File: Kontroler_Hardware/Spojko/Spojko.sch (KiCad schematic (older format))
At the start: 25 parts, among them J1 CONN_01X02, J2 CONN_01X06, P1 Raspberry_Pi, Q1 BSS138, Q2 BSS138, SW1 SW_Reset, SW2 SW_Flash, U1 ESP-12E, U6 DHT11

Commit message: Puno izmena
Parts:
- added V?: VSOURCE, symbol pspice:VSOURCE
- C1, C4, C7: symbol CP -> Spojko-rescue:CP
- C2, C3, C5, C6: symbol C -> Spojko-rescue:C
- J1: symbol CONN_01X02 -> Spojko-rescue:CONN_01X02
- J2: symbol CONN_01X06 -> Spojko-rescue:CONN_01X06
- JP1, JP2: symbol Jumper_NO_Small -> Spojko-rescue:Jumper_NO_Small
- P1: symbol Raspberry_Pi -> Spojko-rescue:Raspberry_Pi
- Q1, Q2: symbol BSS138 -> Spojko-rescue:BSS138
- R1, R2, R3, R4, R5, R6, R9: symbol R -> Spojko-rescue:R
- SW1, SW2: symbol SW_Push -> Spojko-rescue:SW_Push
- U1: symbol ESP-12E -> Spojko-rescue:ESP-12E
- U6: symbol DHT11 -> Spojko-rescue:DHT11
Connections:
- wire segments 99 -> 136
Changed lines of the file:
@@
-EESchema Schematic File Version 2
+EESchema Schematic File Version 4
 LIBS:Spojko-cache
-LIBS:power
-LIBS:device
-LIBS:transistors
-LIBS:conn
-LIBS:linear
-LIBS:regul
-LIBS:74xx
-LIBS:cmos4000
-LIBS:adc-dac
-LIBS:memory
-LIBS:xilinx
-LIBS:microcontrollers
-LIBS:dsp
-LIBS:microchip
-LIBS:analog_switches
-LIBS:motorola
-LIBS:texas
-LIBS:intel
-LIBS:audio
-LIBS:interface
-LIBS:digital-audio
-LIBS:philips
-LIBS:display
-LIBS:cypress
-LIBS:siliconi
-LIBS:opto
-LIBS:atmel
-LIBS:contrib
-LIBS:valves
-LIBS:Symbols_DCDC-ACDC-Converter_RevC_20Jul2012
-LIBS:Symbols_EN60617_13Mar2013
-LIBS:Symbols_EN60617-10_HF-Radio_DRAFT_12Sep2013
-LIBS:Symbols_ICs-Diskrete_RevD10
-LIBS:Symbols_ICs-Opto_RevB_16Sep2013
-LIBS:Symbols_Microcontroller_Philips-NXP_RevA_06Oct2013
-LIBS:Symbols_Socket-DIN41612_RevA
-LIBS:Symbols_Transformer-Diskrete_RevA
-LIBS:SymbolsSimilarEN60617+oldDIN617-RevE8
-LIBS:switches
-LIBS:sensors
-EELAYER 25 0
+EELAYER 26 0
 EELAYER END
 $Descr A4 11693 8268
@@
 $EndSheet
 $Comp
-L Raspberry_Pi P1
+L Spojko-rescue:Raspberry_Pi P1
 U 1 1 5983D0F7
 P 3900 4900
@@
 $EndComp
 $Comp
-L CONN_01X02 J1
+L Spojko-rescue:CONN_01X02 J1
 U 1 1 598505AA
 P 1350 1700
@@
 $EndComp
 $Comp
-L +24V #PWR01
+L Spojko-rescue:+24V #PWR01
 U 1 1 598506CD
 P 1000 1300
@@
 $EndComp
 $Comp
-L +24V #PWR02
+L Spojko-rescue:+24V #PWR02
 U 1 1 598513FD
 P 1850 1050
@@
 GPIO25
 $Comp
-L BSS138 Q2
+L Spojko-rescue:BSS138 Q2
 U 1 1 5988C15D
 P 9000 2900
@@
 SCL
 $Comp
-L BSS138 Q1
+L Spojko-rescue:BSS138 Q1
 U 1 1 5988D7F6
 P 8600 3350
@@
 $EndComp
 $Comp
-L Jumper_NO_Small JP2
+L Spojko-rescue:Jumper_NO_Small JP2
 U 1 1 5988ED75
 P 8200 3000
@@
 $EndComp
 $Comp
-L Jumper_NO_Small JP1
+L Spojko-rescue:Jumper_NO_Small JP1
 U 1 1 5988EE7A
 P 8150 3450
@@
 +5V
 $Comp
-L R R3
+L Spojko-rescue:R R3
 U 1 1 59890105
 P 9400 3200
@@
 $EndComp
 $Comp
-L R R4
+L Spojko-rescue:R R4
 U 1 1 598901B2
 P 9600 2800
@@
 $EndSheet
 $Comp
-L ESP-12E U1
+L Spojko-rescue:ESP-12E U1
 U 1 1 598AF9FB
 P 8750 5000
@@
 $EndComp
 $Comp
-L CP C4
+L Spojko-rescue:CP C4
 U 1 1 598A3011
 P 6650 1200
@@
 $EndComp
 $Comp
-L C C5
+L Spojko-rescue:C C5
 U 1 1 598A30B2
 P 6650 1500
@@
 Spojko napajanja\n
 $Comp
-L SW_Push SW1
+L Spojko-rescue:SW_Push SW1
 U 1 1 598FB508
 P 7100 4700
@@
 $EndComp
 $Comp
-L SW_Push SW2
+L Spojko-rescue:SW_Push SW2
 U 1 1 598FB5DB
 P 10300 5100
@@
 $EndComp
 $Comp
-L R R1
+L Spojko-rescue:R R1
 U 1 1 598FB759
 P 7450 5050
@@
 GND
 $Comp
-L R R2
+L Spojko-rescue:R R2
 U 1 1 598FC9D7
 P 7650 5050
@@
 $EndComp
 $Comp
-L R R6
+L Spojko-rescue:R R6
 U 1 1 598FCC56
 P 10050 5350
@@
 +3V3
 $Comp
-L R R5
+L Spojko-rescue:R R5
 U 1 1 598FD30F
 P 9850 5450
@@
 $EndComp
 $Comp
-L CONN_01X06 J2
+L Spojko-rescue:CONN_01X06 J2
 U 1 1 598FDB37
 P 1700 7200
@@
 Spojko konektor pinout
 $Comp
-L DHT11 U6
+L Spojko-rescue:DHT11 U6
 U 1 1 5990897F
 P 1650 3600
@@
 GND
 $Comp
-L R R9
+L Spojko-rescue:R R9
 U 1 1 5990A619
 P 2100 3800
@@
 Bypass C\nESP
 $Comp
-L CP C1
+L Spojko-rescue:CP C1
 U 1 1 59A73070
 P 5350 1200
@@
 $EndComp
 $Comp
-L C C2
+L Spojko-rescue:C C2
 U 1 1 59A73076
 P 5350 1500
@@
 Bypass C\nMCU
 $Comp
-L C C3
+L Spojko-rescue:C C3
 U 1 1 59A741DA
 P 5350 1800
@@
 $EndComp
 $Comp
-L C C6
+L Spojko-rescue:C C6
 U 1 1 59A775AE
 P 6650 1800
@@
 $EndComp
 $Comp
-L CP C7
+L Spojko-rescue:CP C7
 U 1 1 59A8B614
 P 8050 1500
@@
 	1000 1800 1000 1750
 Wire Wire Line
-	1000 1750 1150 1750
+	1000 1750 1100 1750
 Wire Wire Line
 	3750 1600 3450 1600
@@
 	8300 3000 8800 3000
 Wire Wire Line
-	9200 3000 9750 3000
-Wire Wire Line
-	8800 3450 9750 3450
+	9200 3000 9600 3000
+Wire Wire Line
+	8800 3450 9400 3450
 Wire Wire Line
 	9400 3350 9400 3450
@@
 	9400 3050 9400 2500
 Wire Wire Line
-	9400 2500 9750 2500
+	9400 2500 9600 2500
 Wire Wire Line
 	9600 2650 9600 2500
 Connection ~ 9600 2500
 Wire Wire Line
-	8350 2500 8950 2500
+	8350 2500 8550 2500
 Wire Wire Line
 	8550 2500 8550 3150
@@
 	7450 4900 7450 4700
 Wire Wire Line
-	7300 4700 7850 4700
+	7300 4700 7450 4700
 Connection ~ 7450 4700
 Wire Wire Line
@@
 	9650 5700 9850 5700
 Wire Wire Line
-	9850 5600 9850 5850
+	9850 5600 9850 5700
 Connection ~ 9850 5700
 Wire Wire Line
@@
 	10850 1050 8750 1050
 Wire Wire Line
-	1950 3500 2450 3500
-Wire Wire Line
-	2350 3900 2350 4700
+	1950 3500 2100 3500
+Wire Wire Line
+	2350 3900 2350 3950
 Wire Wire Line
 	2350 3950 2350 3850
@@
 	2100 3950 1650 3950
 Wire Wire Line
-	1650 3900 1650 4150
+	1650 3900 1650 3950
 Connection ~ 1650 3950
 Wire Wire Line
@@
 	5200 1200 5150 1200
 Wire Wire Line
-	5150 1200 5150 1800
+	5150 1200 5150 1500
 Wire Wire Line
 	5150 1800 5200 1800
 Wire Wire Line
-	5050 1500 5200 1500
+	5050 1500 5150 1500
 Connection ~ 5150 1500
 Wire Wire Line
 	5500 1200 5550 1200
 Wire Wire Line
-	5550 1200 5550 1800
+	5550 1200 5550 1500
 Wire Wire Line
 	5550 1800 5500 1800
 Wire Wire Line
-	5500 1500 5650 1500
+	5500 1500 5550 1500
 Connection ~ 5550 1500
 Wire Wire Line
 	6500 1200 6450 1200
 Wire Wire Line
-	6450 1200 6450 1800
+	6450 1200 6450 1500
 Wire Wire Line
 	6450 1800 6500 1800
 Wire Wire Line
-	6350 1500 6500 1500
+	6350 1500 6450 1500
 Connection ~ 6450 1500
 Wire Wire Line
 	6800 1200 6850 1200
 Wire Wire Line
-	6850 1200 6850 1800
+	6850 1200 6850 1500
 Wire Wire Line
 	6850 1800 6800 1800
 Wire Wire Line
-	6800 1500 6950 1500
+	6800 1500 6850 1500
 Connection ~ 6850 1500
 Wire Wire Line
@@
 	8200 1500 8350 1500
 Wire Wire Line
-	2200 3150 2450 3150
+	2200 3150 2300 3150
 Wire Wire Line
 	2300 3250 2300 3150
@@
 	2000 1150 1850 1150
 Wire Wire Line
-	1850 1050 1850 2050
+	1850 1050 1850 1150
 Wire Wire Line
 	1850 2050 2000 2050
@@
 	6950 5200 7850 5200
 Wire Wire Line
-	6850 5400 7850 5400
+	6850 5400 7450 5400
 Wire Wire Line
 	10500 5100 10600 5100
@@
 Wire Wire Line
 	5150 4200 5000 4200
+Wire Wire Line
+	2350 3950 2350 4050
+Wire Wire Line
+	2350 4050 2350 4150
+Wire Wire Line
+	2350 4150 2350 4250
+Wire Wire Line
+	2350 4250 2350 4350
+Wire Wire Line
+	2350 4350 2350 4450
+Wire Wire Line
+	2350 4450 2350 4550
+Wire Wire Line
+	2350 4550 2350 4700
+Wire Wire Line
+	9400 3450 9750 3450
+Wire Wire Line
+	9600 3000 9750 3000
+Wire Wire Line
+	9600 2500 9750 2500
+Wire Wire Line
+	8550 2500 8950 2500
+Wire Wire Line
+	7450 5400 7650 5400
+Wire Wire Line
+	7450 4700 7850 4700
+Wire Wire Line
+	7650 5400 7850 5400
+Wire Wire Line
+	9850 5700 9850 5850
+Wire Wire Line
+	2100 3500 2450 3500
+Wire Wire Line
+	1650 3950 1650 4150
+Wire Wire Line
+	5150 1500 5150 1800
+Wire Wire Line
+	5150 1500 5200 1500
+Wire Wire Line
+	5550 1500 5550 1800
+Wire Wire Line
+	5550 1500 5650 1500
+Wire Wire Line
+	6450 1500 6450 1800
+Wire Wire Line
+	6450 1500 6500 1500
+Wire Wire Line
+	6850 1500 6850 1800
+Wire Wire Line
+	6850 1500 6950 1500
+Wire Wire Line
+	2300 3150 2450 3150
+Wire Wire Line
+	1850 1150 1850 1600
+Wire Wire Line
+	1850 1600 1850 2050
+$Comp
+L pspice:VSOURCE V?
+U 1 1 5ADCA63F
+P 900 2850
+F 0 "V?" H 1128 2896 50  0000 L CNN
+F 1 "VSOURCE" H 1128 2805 50  0000 L CNN
+F 2 "" H 900 2850 50  0001 C CNN
+F 3 "" H 900 2850 50  0001 C CNN
+	1    900  2850
+	1    0    0    -1
+$EndComp
+Wire Wire Line
+	1000 1650 900  1650
+Wire Wire Line
+	900  1650 900  2550
+Connection ~ 1000 1650
+Wire Wire Line
+	900  3150 1500 3150
+Wire Wire Line
+	1500 3150 1500 2300
+Wire Wire Line
+	1500 2300 1200 2300
+Wire Wire Line
+	1200 2300 1200 1850
+Wire Wire Line
+	1200 1850 1100 1850
+Wire Wire Line
+	1100 1850 1100 1750
+Connection ~ 1100 1750
+Wire Wire Line
+	1100 1750 1150 1750
 $EndSCHEMATC

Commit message: Deleted  PCB Spojko
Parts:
- removed V?: VSOURCE, symbol pspice:VSOURCE
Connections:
- wire segments 136 -> 127
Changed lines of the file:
@@
 	1000 1800 1000 1750
-Wire Wire Line
-	1000 1750 1100 1750
 Wire Wire Line
 	3750 1600 3450 1600
@@
 Wire Wire Line
 	1850 1600 1850 2050
-$Comp
-L pspice:VSOURCE V?
-U 1 1 5ADCA63F
-P 900 2850
-F 0 "V?" H 1128 2896 50  0000 L CNN
-F 1 "VSOURCE" H 1128 2805 50  0000 L CNN
-F 2 "" H 900 2850 50  0001 C CNN
-F 3 "" H 900 2850 50  0001 C CNN
-	1    900  2850
-	1    0    0    -1
-$EndComp
-Wire Wire Line
-	1000 1650 900  1650
-Wire Wire Line
-	900  1650 900  2550
-Connection ~ 1000 1650
-Wire Wire Line
-	900  3150 1500 3150
-Wire Wire Line
-	1500 3150 1500 2300
-Wire Wire Line
-	1500 2300 1200 2300
-Wire Wire Line
-	1200 2300 1200 1850
-Wire Wire Line
-	1200 1850 1100 1850
-Wire Wire Line
-	1100 1850 1100 1750
-Connection ~ 1100 1750
-Wire Wire Line
-	1100 1750 1150 1750
+Wire Wire Line
+	1000 1750 1150 1750
 $EndSCHEMATC

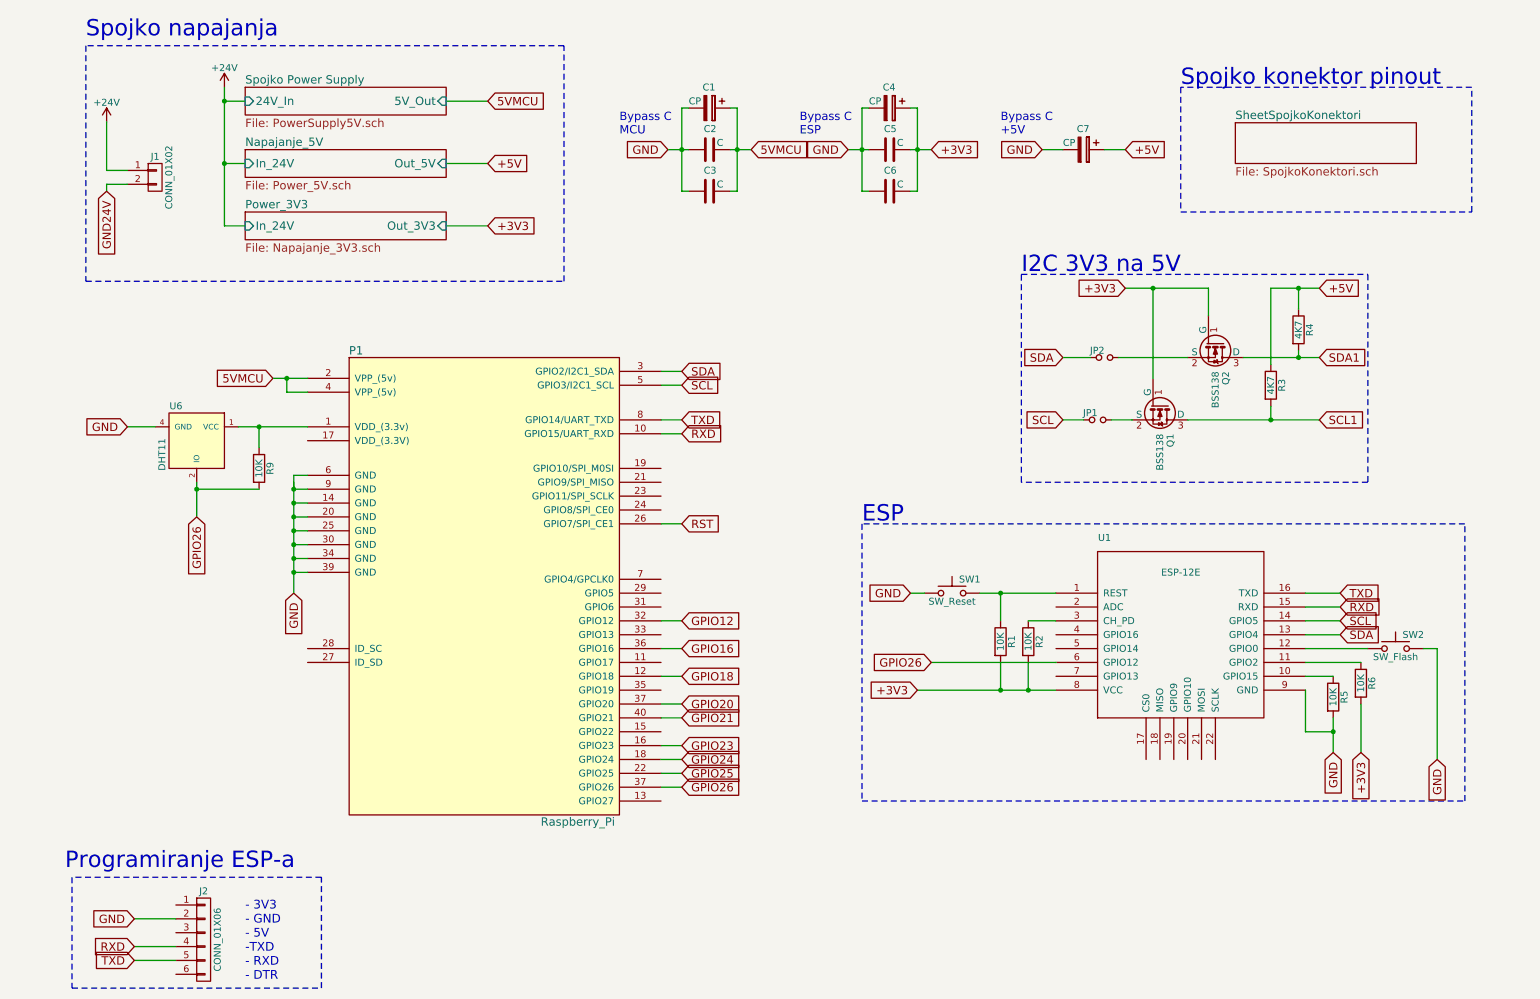
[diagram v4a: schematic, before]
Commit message: NewTemplates
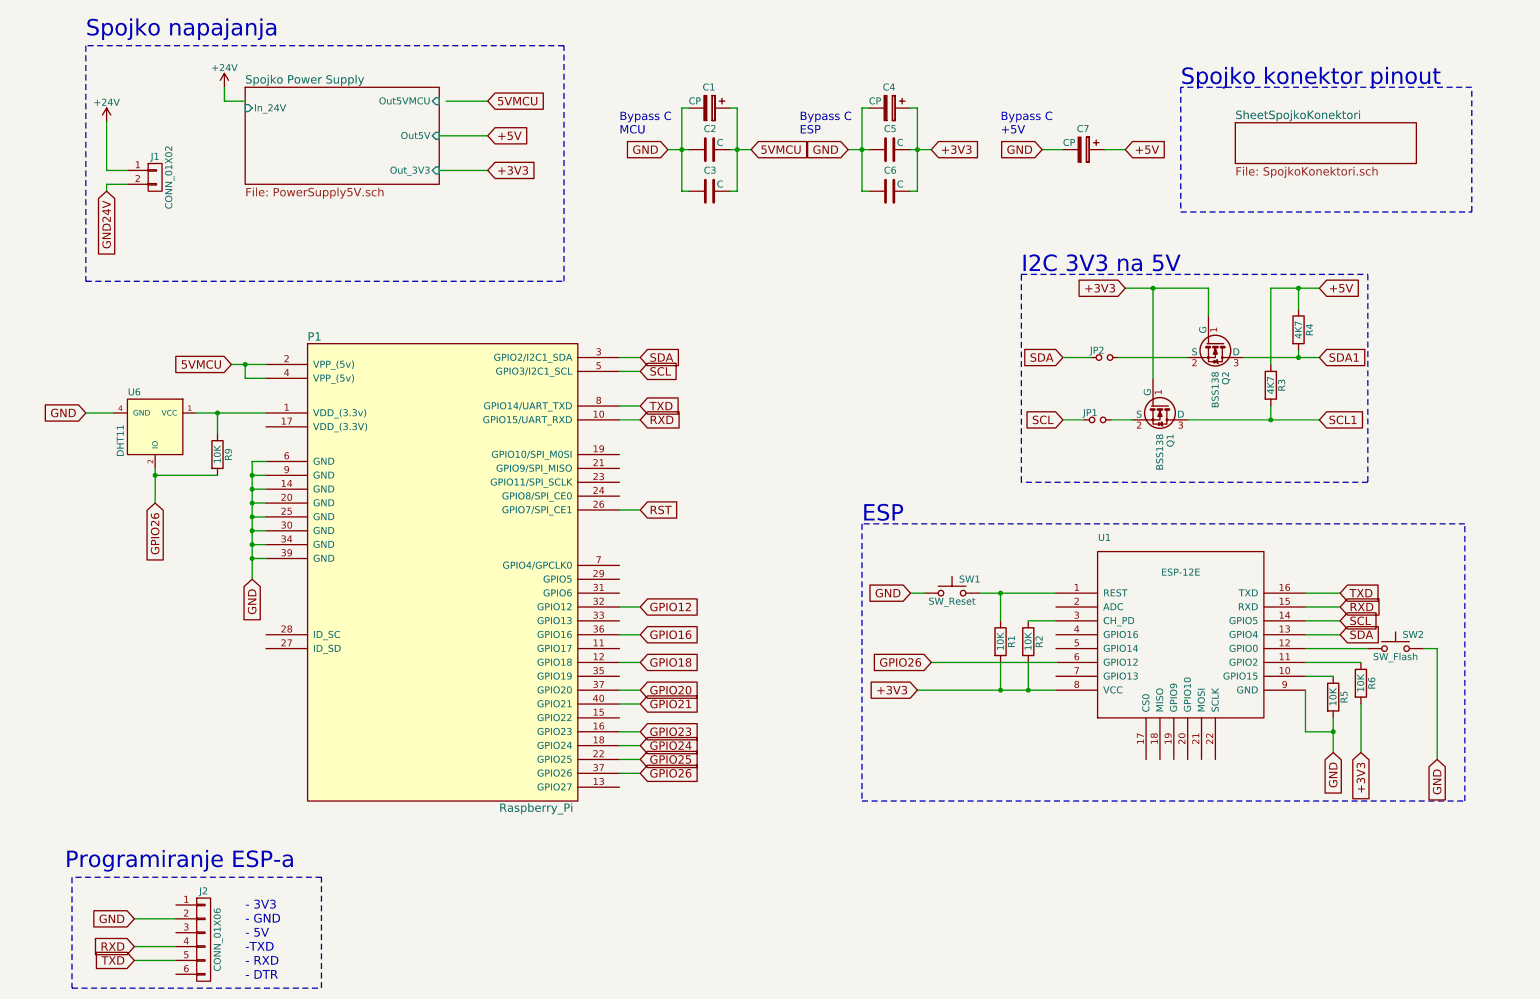
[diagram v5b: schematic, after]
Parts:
- P1: footprint Pin_Headers:Pin_Header_Straight_2x20_Pitch2.54mm -> Connector_PinHeader_2.54mm:PinHeader_2x20_P2.54mm_Vertical
- Q1, Q2: footprint TO_SOT_Packages_SMD:SOT-23 -> Package_TO_SOT_SMD:SOT-23
- R1, R2: footprint Resistors_SMD:R_1206 -> Resistor_SMD:R_1206_3216Metric
- R5: footprint Resistors_SMD:R_0805 -> Resistor_SMD:R_0805_2012Metric
- U1: footprint project_footprints:ESP-12E -> lib_fp:ESP-12E
- U6: footprint project_footprints:DHT22_Temperature_Humidity -> lib_fp:DHT22_Temperature_Humidity
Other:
- moved on the sheet: P1, R9, U6
